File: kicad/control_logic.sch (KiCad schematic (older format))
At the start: 32 parts, among them U108 74HC04, U109 74HC04, U110 74HC04, U111 74HC04, U112 74LS574, U113 SST39SF040, U114 74HC04, U115 74HC04, U117 74LS08, U118 74HC245, U125 74HC04, U87 74LS574, U88 SST39SF040, U89 74LS574, U90 SST39SF040, U92 74LS154

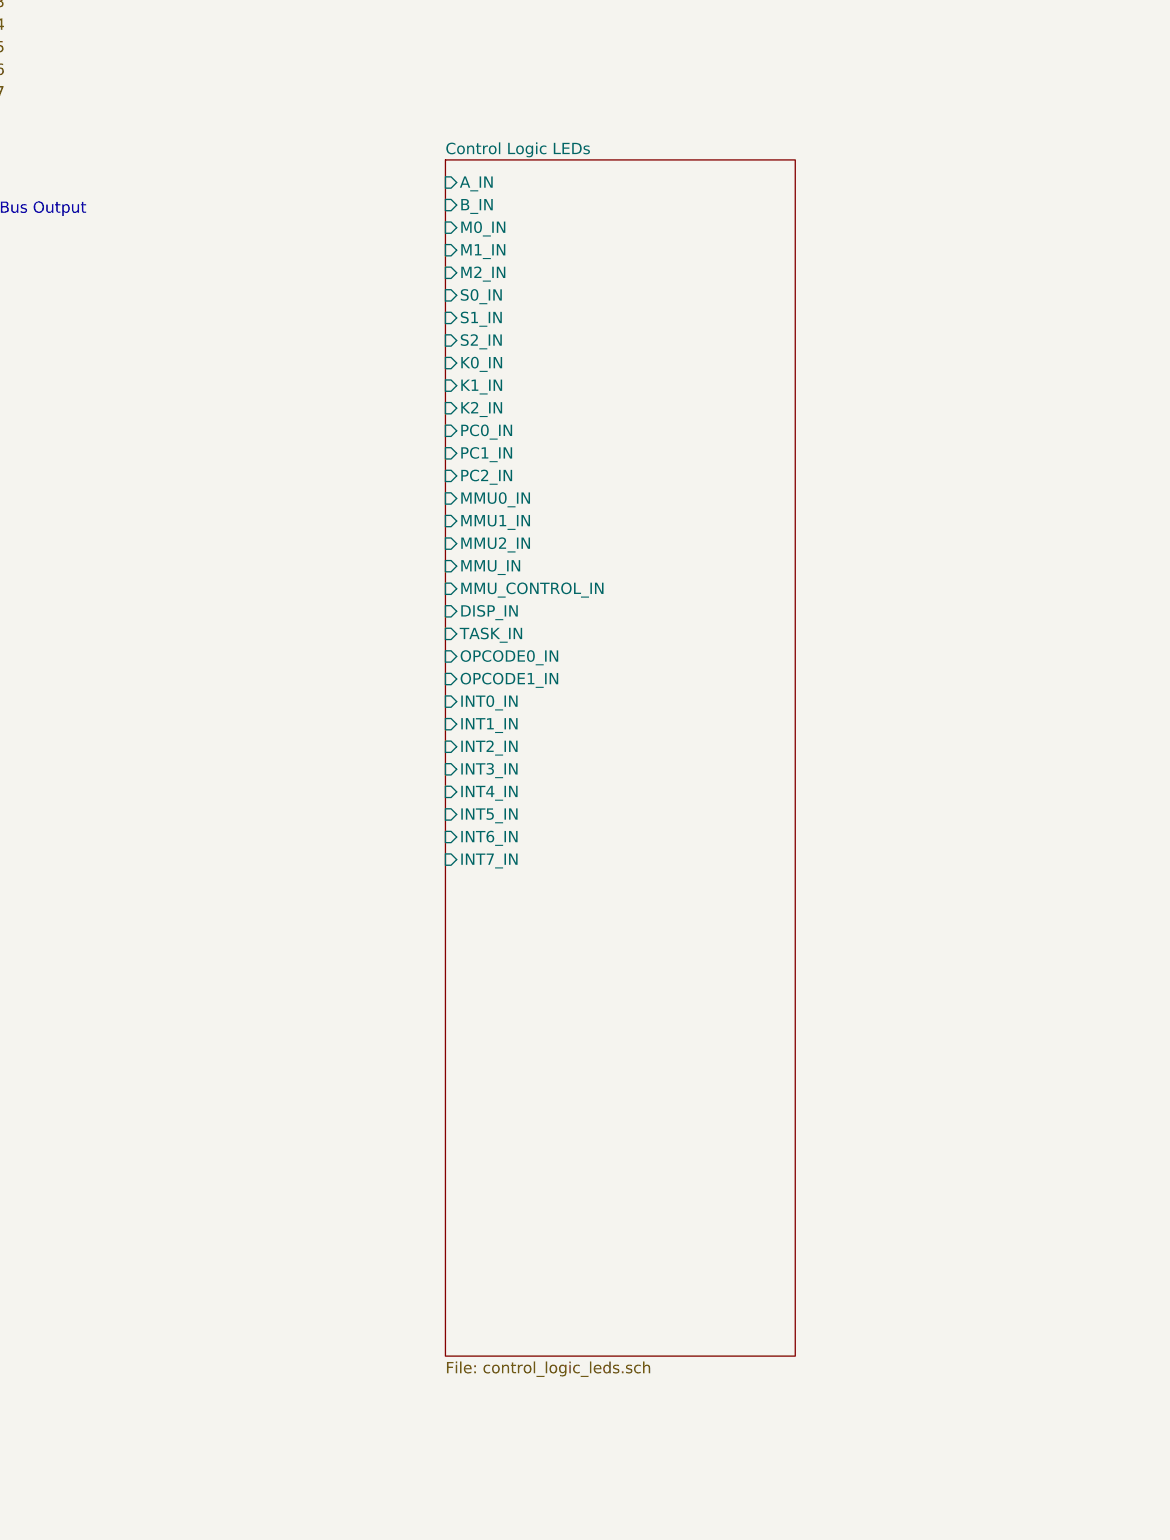
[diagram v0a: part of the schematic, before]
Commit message: Going to try out resistor network.
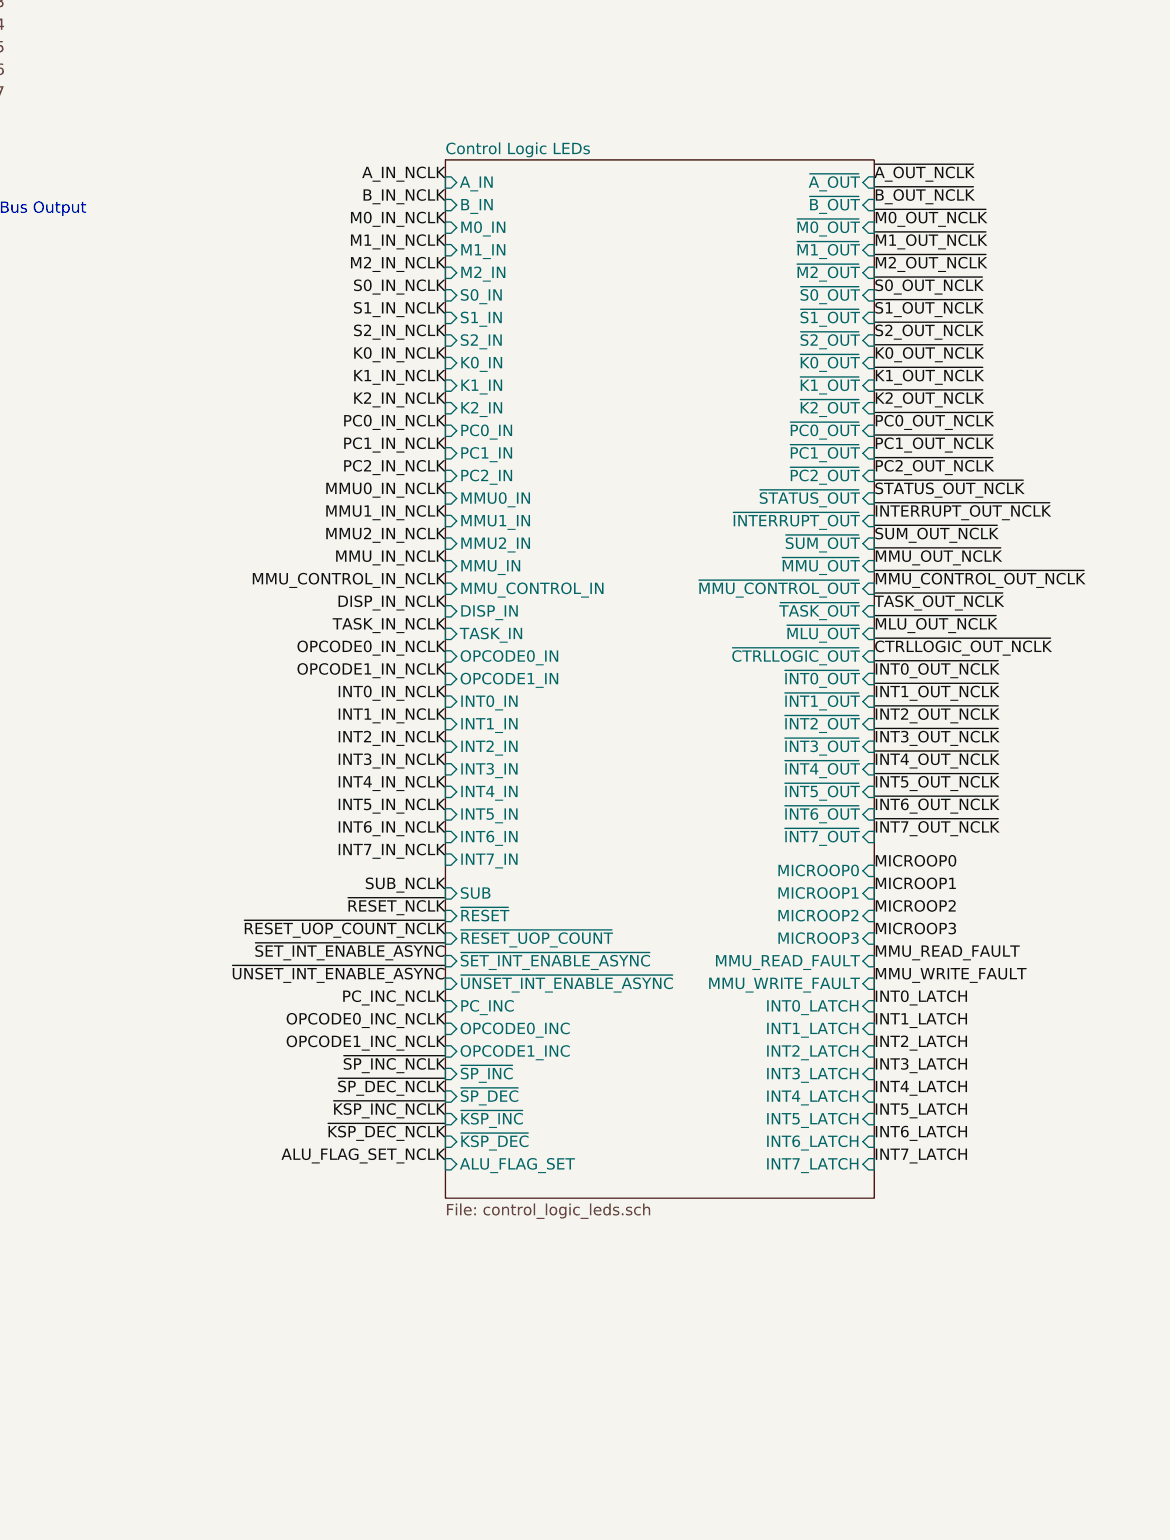
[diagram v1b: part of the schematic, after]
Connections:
- net labels added: OPCODE0_IN_NCLK, OPCODE1_IN_NCLK, PC0_IN_NCLK, PC1_IN_NCLK, PC2_IN_NCLK
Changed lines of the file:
@@
 $EndComp
 $Sheet
-S 18450 4150 1550 5300
+S 18450 4150 1900 4600
 U 5B1644E8
 F0 "Control Logic LEDs" 50
@@
 F31 "INT6_IN" I L 18450 7150 50
 F32 "INT7_IN" I L 18450 7250 50
+F33 "~A_OUT" I R 20350 4250 50
+F34 "~B_OUT" I R 20350 4350 50
+F35 "~M0_OUT" I R 20350 4450 50
+F36 "~M1_OUT" I R 20350 4550 50
+F37 "~M2_OUT" I R 20350 4650 50
+F38 "~S0_OUT" I R 20350 4750 50
+F39 "~S1_OUT" I R 20350 4850 50
+F40 "~S2_OUT" I R 20350 4950 50
+F41 "~K0_OUT" I R 20350 5050 50
+F42 "~K1_OUT" I R 20350 5150 50
+F43 "~K2_OUT" I R 20350 5250 50
+F44 "~PC0_OUT" I R 20350 5350 50
+F45 "~PC1_OUT" I R 20350 5450 50
+F46 "~PC2_OUT" I R 20350 5550 50
+F47 "~STATUS_OUT" I R 20350 5650 50
+F48 "~INTERRUPT_OUT" I R 20350 5750 50
+F49 "~SUM_OUT" I R 20350 5850 50
+F50 "~MMU_OUT" I R 20350 5950 50
+F51 "~MMU_CONTROL_OUT" I R 20350 6050 50
+F52 "~TASK_OUT" I R 20350 6150 50
+F53 "~MLU_OUT" I R 20350 6250 50
+F54 "~CTRLLOGIC_OUT" I R 20350 6350 50
+F55 "~INT1_OUT" I R 20350 6550 50
+F56 "~INT2_OUT" I R 20350 6650 50
+F57 "~INT3_OUT" I R 20350 6750 50
+F58 "~INT4_OUT" I R 20350 6850 50
+F59 "~INT5_OUT" I R 20350 6950 50
+F60 "~INT6_OUT" I R 20350 7050 50
+F61 "~INT7_OUT" I R 20350 7150 50
+F62 "~INT0_OUT" I R 20350 6450 50
+F63 "SUB" I L 18450 7400 50
+F64 "~RESET" I L 18450 7500 50
+F65 "~RESET_UOP_COUNT" I L 18450 7600 50
+F66 "~SET_INT_ENABLE_ASYNC" I L 18450 7700 50
+F67 "~UNSET_INT_ENABLE_ASYNC" I L 18450 7800 50
+F68 "PC_INC" I L 18450 7900 50
+F69 "OPCODE0_INC" I L 18450 8000 50
+F70 "OPCODE1_INC" I L 18450 8100 50
+F71 "~SP_INC" I L 18450 8200 50
+F72 "~SP_DEC" I L 18450 8300 50
+F73 "~KSP_INC" I L 18450 8400 50
+F74 "~KSP_DEC" I L 18450 8500 50
+F75 "ALU_FLAG_SET" I L 18450 8600 50
+F76 "MICROOP0" I R 20350 7300 50
+F77 "MICROOP1" I R 20350 7400 50
+F78 "MICROOP2" I R 20350 7500 50
+F79 "MICROOP3" I R 20350 7600 50
+F80 "MMU_READ_FAULT" I R 20350 7700 50
+F81 "MMU_WRITE_FAULT" I R 20350 7800 50
+F82 "INT0_LATCH" I R 20350 7900 50
+F83 "INT1_LATCH" I R 20350 8000 50
+F84 "INT2_LATCH" I R 20350 8100 50
+F85 "INT3_LATCH" I R 20350 8200 50
+F86 "INT4_LATCH" I R 20350 8300 50
+F87 "INT5_LATCH" I R 20350 8400 50
+F88 "INT6_LATCH" I R 20350 8500 50
+F89 "INT7_LATCH" I R 20350 8600 50
 $EndSheet
 Text Notes 7150 5550 0    79   ~ 0
 TODO: Connect these and INs, \nand interrupt lines up to\nboard interconnect.\n
+Text Label 18450 4250 2    50   ~ 0
+A_IN_NCLK
+Text Label 18450 4350 2    50   ~ 0
+B_IN_NCLK
+Text Label 18450 4450 2    50   ~ 0
+M0_IN_NCLK
+Text Label 18450 4550 2    50   ~ 0
+M1_IN_NCLK
+Text Label 18450 4650 2    50   ~ 0
+M2_IN_NCLK
+Text Label 18450 4750 2    50   ~ 0
+S0_IN_NCLK
+Text Label 18450 4850 2    50   ~ 0
+S1_IN_NCLK
+Text Label 18450 4950 2    50   ~ 0
+S2_IN_NCLK
+Text Label 18450 5050 2    50   ~ 0
+K0_IN_NCLK
+Text Label 18450 5150 2    50   ~ 0
+K1_IN_NCLK
+Text Label 18450 5250 2    50   ~ 0
+K2_IN_NCLK
+Text Label 18450 5350 2    50   ~ 0
+PC0_IN_NCLK
+Text Label 18450 5450 2    50   ~ 0
+PC1_IN_NCLK
+Text Label 18450 5550 2    50   ~ 0
+PC2_IN_NCLK
+Text Label 18450 5650 2    50   ~ 0
+MMU0_IN_NCLK
+Text Label 18450 5750 2    50   ~ 0
+MMU1_IN_NCLK
+Text Label 18450 5850 2    50   ~ 0
+MMU2_IN_NCLK
+Text Label 18450 5950 2    50   ~ 0
+MMU_IN_NCLK
+Text Label 18450 6050 2    50   ~ 0
+MMU_CONTROL_IN_NCLK
+Text Label 18450 6150 2    50   ~ 0
+DISP_IN_NCLK
+Text Label 18450 6250 2    50   ~ 0
+TASK_IN_NCLK
+Text Label 18450 6350 2    50   ~ 0
+OPCODE0_IN_NCLK
+Text Label 18450 6450 2    50   ~ 0
+OPCODE1_IN_NCLK
+Text Label 18450 6550 2    50   ~ 0
+INT0_IN_NCLK
+Text Label 18450 6650 2    50   ~ 0
+INT1_IN_NCLK
+Text Label 18450 6750 2    50   ~ 0
+INT2_IN_NCLK
+Text Label 18450 6850 2    50   ~ 0
+INT3_IN_NCLK
+Text Label 18450 6950 2    50   ~ 0
+INT4_IN_NCLK
+Text Label 18450 7050 2    50   ~ 0
+INT5_IN_NCLK
+Text Label 18450 7150 2    50   ~ 0
+INT6_IN_NCLK
+Text Label 18450 7250 2    50   ~ 0
+INT7_IN_NCLK
+Text Label 20350 4250 0    50   ~ 0
+~A_OUT_NCLK
+Text Label 20350 4350 0    50   ~ 0
+~B_OUT_NCLK
+Text Label 20350 4450 0    50   ~ 0
+~M0_OUT_NCLK
+Text Label 20350 4550 0    50   ~ 0
+~M1_OUT_NCLK
+Text Label 20350 4650 0    50   ~ 0
+~M2_OUT_NCLK
+Text Label 20350 4750 0    50   ~ 0
+~S0_OUT_NCLK
+Text Label 20350 4850 0    50   ~ 0
+~S1_OUT_NCLK
+Text Label 20350 4950 0    50   ~ 0
+~S2_OUT_NCLK
+Text Label 20350 5050 0    50   ~ 0
+~K0_OUT_NCLK
+Text Label 20350 5150 0    50   ~ 0
+~K1_OUT_NCLK
+Text Label 20350 5250 0    50   ~ 0
+~K2_OUT_NCLK
+Text Label 20350 5350 0    50   ~ 0
+~PC0_OUT_NCLK
+Text Label 20350 5450 0    50   ~ 0
+~PC1_OUT_NCLK
+Text Label 20350 5550 0    50   ~ 0
+~PC2_OUT_NCLK
+Text Label 20350 5650 0    50   ~ 0
+~STATUS_OUT_NCLK
+Text Label 20350 5750 0    50   ~ 0
+~INTERRUPT_OUT_NCLK
+Text Label 20350 5850 0    50   ~ 0
+~SUM_OUT_NCLK
+Text Label 20350 5950 0    50   ~ 0
+~MMU_OUT_NCLK
+Text Label 20350 6050 0    50   ~ 0
+~MMU_CONTROL_OUT_NCLK
+Text Label 20350 6150 0    50   ~ 0
+~TASK_OUT_NCLK
+Text Label 20350 6250 0    50   ~ 0
+~MLU_OUT_NCLK
+Text Label 20350 6350 0    50   ~ 0
+~CTRLLOGIC_OUT_NCLK
+Text Label 20350 6450 0    50   ~ 0
+~INT0_OUT_NCLK
+Text Label 20350 6550 0    50   ~ 0
+~INT1_OUT_NCLK
+Text Label 20350 6650 0    50   ~ 0
+~INT2_OUT_NCLK
+Text Label 20350 6750 0    50   ~ 0
+~INT3_OUT_NCLK
+Text Label 20350 6850 0    50   ~ 0
+~INT4_OUT_NCLK
+Text Label 20350 6950 0    50   ~ 0
+~INT5_OUT_NCLK
+Text Label 20350 7050 0    50   ~ 0
+~INT6_OUT_NCLK
+Text Label 20350 7150 0    50   ~ 0
+~INT7_OUT_NCLK
+Text Label 18450 7400 2    50   ~ 0
+SUB_NCLK
+Text Label 18450 7500 2    50   ~ 0
+~RESET_NCLK
+Text Label 18450 7600 2    50   ~ 0
+~RESET_UOP_COUNT_NCLK
+Text Label 18450 7700 2    50   ~ 0
+~SET_INT_ENABLE_ASYNC
+Text Label 18450 7800 2    50   ~ 0
+~UNSET_INT_ENABLE_ASYNC
+Text Label 18450 7900 2    50   ~ 0
+PC_INC_NCLK
+Text Label 18450 8000 2    50   ~ 0
+OPCODE0_INC_NCLK
+Text Label 18450 8100 2    50   ~ 0
+OPCODE1_INC_NCLK
+Text Label 18450 8200 2    50   ~ 0
+~SP_INC_NCLK
+Text Label 18450 8300 2    50   ~ 0
+~SP_DEC_NCLK
+Text Label 18450 8400 2    50   ~ 0
+~KSP_INC_NCLK
+Text Label 18450 8500 2    50   ~ 0
+~KSP_DEC_NCLK
+Text Label 18450 8600 2    50   ~ 0
+ALU_FLAG_SET_NCLK
+Text Label 20350 7300 0    50   ~ 0
+MICROOP0
+Text Label 20350 7400 0    50   ~ 0
+MICROOP1
+Text Label 20350 7500 0    50   ~ 0
+MICROOP2
+Text Label 20350 7600 0    50   ~ 0
+MICROOP3
+Text Label 20350 7700 0    50   ~ 0
+MMU_READ_FAULT
+Text Label 20350 7800 0    50   ~ 0
+MMU_WRITE_FAULT
+Text Label 20350 7900 0    50   ~ 0
+INT0_LATCH
+Text Label 20350 8000 0    50   ~ 0
+INT1_LATCH
+Text Label 20350 8100 0    50   ~ 0
+INT2_LATCH
+Text Label 20350 8200 0    50   ~ 0
+INT3_LATCH
+Text Label 20350 8300 0    50   ~ 0
+INT4_LATCH
+Text Label 20350 8400 0    50   ~ 0
+INT5_LATCH
+Text Label 20350 8500 0    50   ~ 0
+INT6_LATCH
+Text Label 20350 8600 0    50   ~ 0
+INT7_LATCH
 $EndSCHEMATC
